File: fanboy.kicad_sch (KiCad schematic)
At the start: 51 parts, among them J1 XT30, J2 USB_C_Receptacle_USB2.0, J3 Conn_01x04, J4 Conn_01x04, SW1 GT-TC029B-H025-L1N, SW2 GT-TC029B-H025-L1N, U1 TPD1E05U06DYA, U2 TPD1E05U06DYA, U3 W25Q16JVUXIQ TR, U4 TLV1117LV33DCYR, U5 EMC2302, U6 RP2040, U7 SK6812, Y1 12MHz

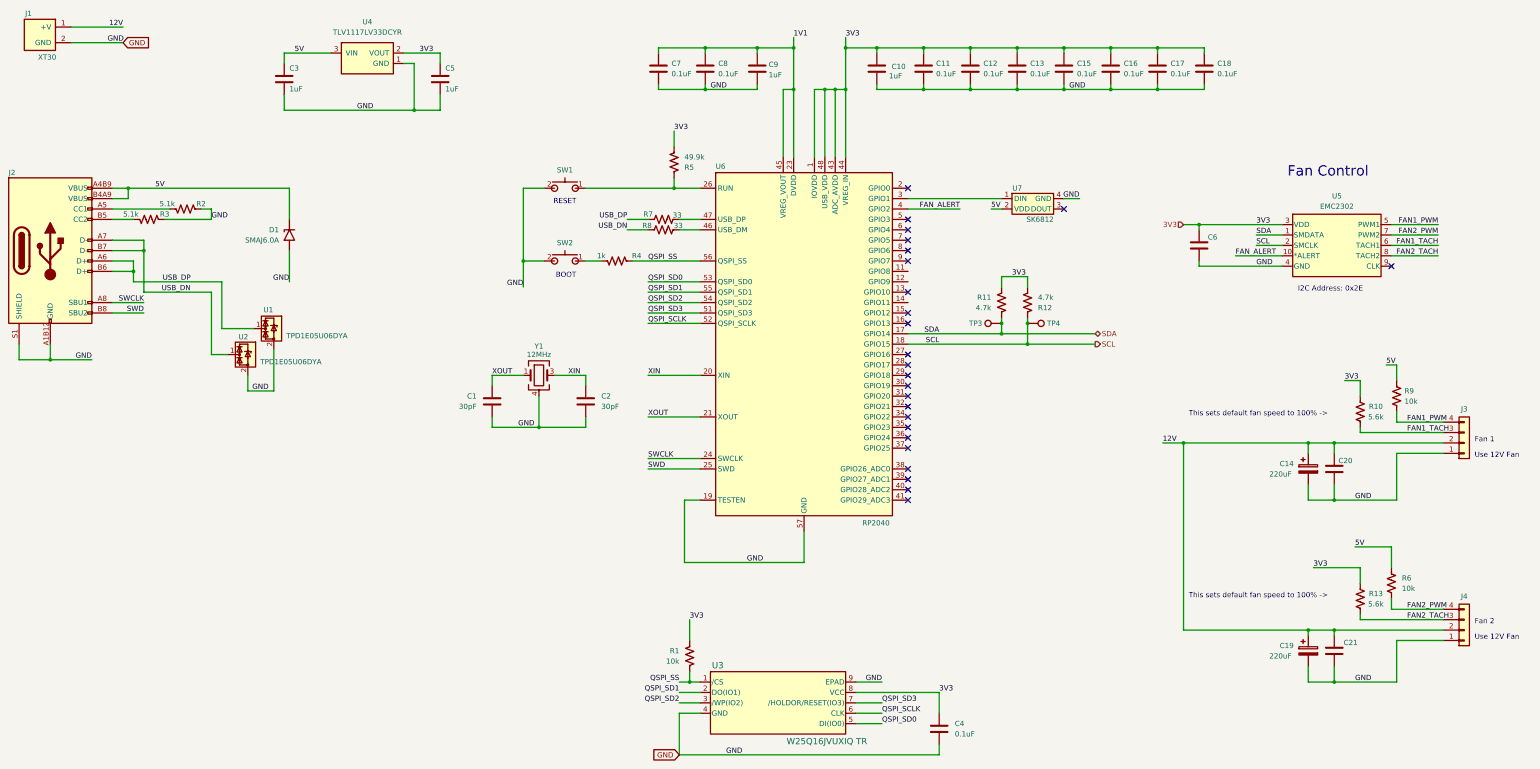
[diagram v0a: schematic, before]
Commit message: finished routing, added render and readme
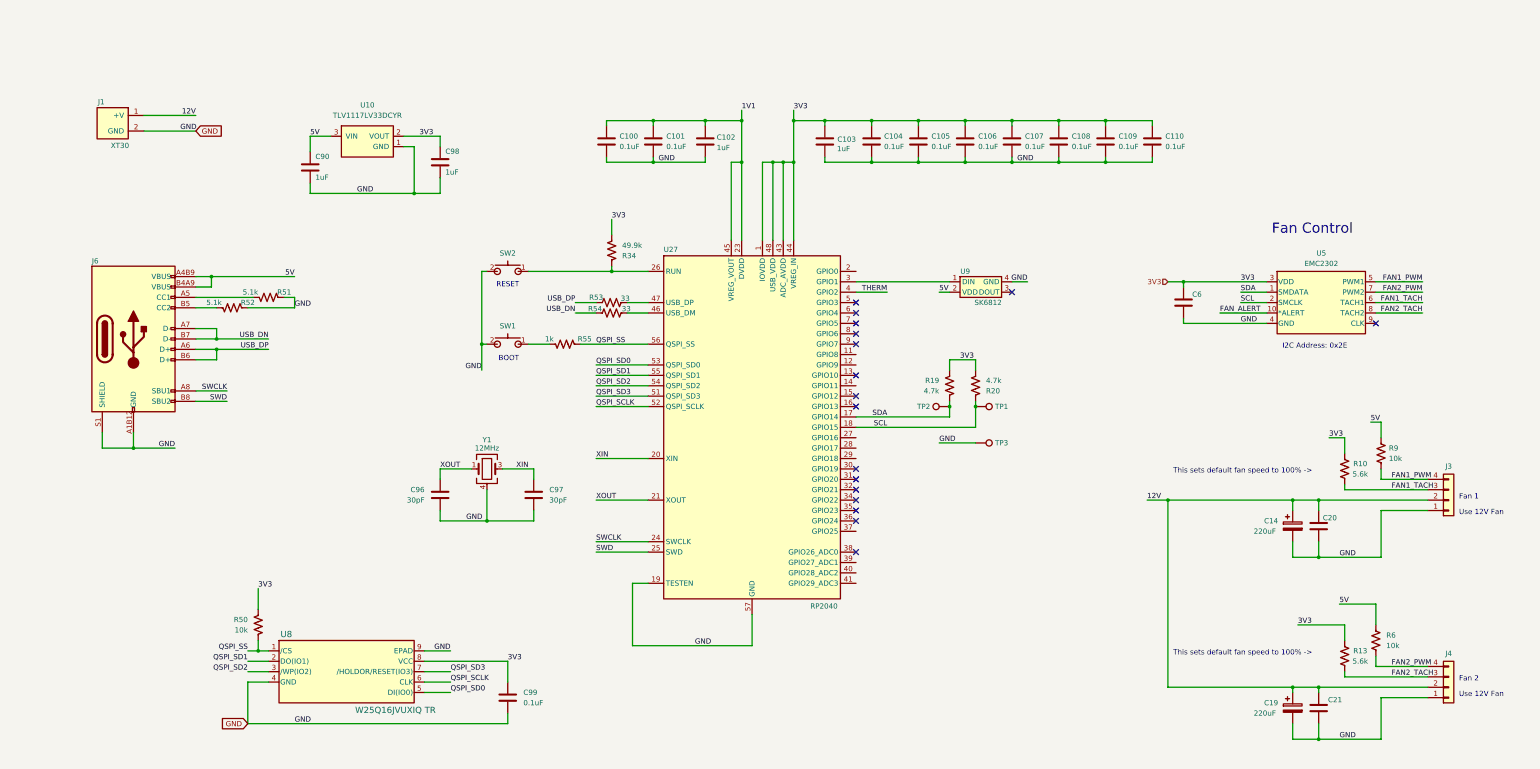
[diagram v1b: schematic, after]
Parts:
- removed C1, C2: 30pF, Capacitor_SMD:C_0402_1005Metric, symbol Device:C
- removed C10, C3, C5, C9: 1uF, Capacitor_SMD:C_0402_1005Metric, symbol Device:C
- removed C11, C12, C13, C15, C16, C17, C18, C4, C7, C8: 0.1uF, Capacitor_SMD:C_0402_1005Metric, symbol Device:C
- removed D1: SMAJ6.0A, Diode_SMD:D_SMB, symbol Diode:SMAJ6.0A
- removed J2: USB_C_Receptacle_USB2.0, aditBoard:USB_C_Receptacle_GCT_USB4105-xx-A_16P_TopMnt_Horizontal, symbol aditBoard:USB_C_Receptacle_USB2.0
- removed R1: 10k, Resistor_SMD:R_0402_1005Metric, symbol Device:R_US
- removed R11, R12: 4.7k, Resistor_SMD:R_0402_1005Metric, symbol Device:R_US
- removed R2, R3: 5.1k, Resistor_SMD:R_0402_1005Metric, symbol Device:R_US
- removed R4: 1k, Resistor_SMD:R_0402_1005Metric, symbol Device:R_US
- removed R5: 49.9k, Resistor_SMD:R_0402_1005Metric, symbol Device:R_US
- removed R7, R8: 33, Resistor_SMD:R_0402_1005Metric, symbol Device:R_US
- removed TP4: TestPoint, TestPoint:TestPoint_Pad_D1.0mm, symbol Connector:TestPoint
- removed U1, U2: TPD1E05U06DYA, Diode_SMD:D_SOD-523, symbol Power_Protection:TPD1E05U06DYA
- removed U3: W25Q16JVUXIQ TR, emberone:USON-8_UX_2x3x0p6_WIN, symbol emberone:W25Q16JVUXIQ_TR
- removed U4: TLV1117LV33DCYR, emberone:VREG_TLV1117LV33DCYR, symbol emberone:TLV1117LV33DCYR
- removed U6: RP2040, Package_DFN_QFN:QFN-56-1EP_7x7mm_P0.4mm_EP3.2x3.2mm, symbol aditBoard:RP2040
- removed U7: SK6812, emberone:LED-SMD_4P-L4.0-W1.6-L, symbol athvfd:SK6812SIDE-A-RVS
- added C100, C101, C104, C105, C106, C107, C108, C109, C110, C99: 0.1uF, Capacitor_SMD:C_0402_1005Metric, symbol Device:C
- added C102, C103, C90, C98: 1uF, Capacitor_SMD:C_0402_1005Metric, symbol Device:C
- added C96, C97: 30pF, Capacitor_SMD:C_0402_1005Metric, symbol Device:C
- added J6: USB_C_Receptacle_USB2.0, aditBoard:USB_C_Receptacle_GCT_USB4105-xx-A_16P_TopMnt_Horizontal, symbol aditBoard:USB_C_Receptacle_USB2.0
- added R19, R20: 4.7k, Resistor_SMD:R_0402_1005Metric, symbol Device:R_US
- added R34: 49.9k, Resistor_SMD:R_0402_1005Metric, symbol Device:R_US
- added R50: 10k, Resistor_SMD:R_0402_1005Metric, symbol Device:R_US
- added R51, R52: 5.1k, Resistor_SMD:R_0402_1005Metric, symbol Device:R_US
- added R53, R54: 33, Resistor_SMD:R_0402_1005Metric, symbol Device:R_US
- added R55: 1k, Resistor_SMD:R_0402_1005Metric, symbol Device:R_US
- added TP1, TP2: TestPoint, TestPoint:TestPoint_Pad_D1.0mm, symbol Connector:TestPoint
- added U10: TLV1117LV33DCYR, emberone:VREG_TLV1117LV33DCYR, symbol emberone:TLV1117LV33DCYR
- added U27: RP2040, Package_DFN_QFN:QFN-56-1EP_7x7mm_P0.4mm_EP3.2x3.2mm, symbol aditBoard:RP2040
- added U8: W25Q16JVUXIQ TR, emberone:USON-8_UX_2x3x0p6_WIN, symbol emberone:W25Q16JVUXIQ_TR
- added U9: SK6812, emberone:LED-SMD_4P-L4.0-W1.6-L, symbol athvfd:SK6812SIDE-A-RVS
- renumbered SW2 to SW1, SW1 to SW2
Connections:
- net 1V1: now also C100.2, C101.2, C102.2, U27.23 (DVDD), U27.45 (VREG_VOUT), U27.50 (DVDD)
- net 3V3: now also C103.2, C104.2, C105.2, C106.2, C107.2, C108.2, C109.2, C110.2, C98.1, C99.2, R19.1, R20.2, R34.2, R50.1, U10.2 (VOUT), U10.4 (VOUT), U27.1 (IOVDD), U27.10 (IOVDD), U27.22 (IOVDD), U27.33 (IOVDD), U27.42 (IOVDD), U27.43 (ADC_AVDD), U27.44 (VREG_IN), U27.48 (USB_VDD), U27.49 (IOVDD), U8.8 (VCC)
- net 5V: now also C90.1, J6.A4B9 (VBUS), J6.B4A9 (VBUS), U10.3 (VIN), U9.2 (VDD)
- net GND: now also TP3.1, C100.1, C101.1, C102.1, C103.1, C104.1, C105.1, C106.1, C107.1, C108.1, C109.1, C110.1, C90.2, C96.1, C97.1, C98.2, C99.1, J6.A1B12 (GND), J6.B1A12 (GND), J6.S1 (SHIELD), R51.1, R52.1, U10.1 (GND), U27.19 (TESTEN), U27.57 (GND), U8.4 (GND), U8.9 (EPAD), U9.4 (GND)
- net QSPI_SCLK: now also U27.52 (QSPI_SCLK), U8.6 (CLK)
- net QSPI_SD0: now also U27.53 (QSPI_SD0), U8.5 (DI(IO0))
- net QSPI_SD1: now also U27.55 (QSPI_SD1), U8.2 (DO(IO1))
- net QSPI_SD2: now also U27.54 (QSPI_SD2), U8.3 (/WP(IO2))
- net QSPI_SD3: now also U27.51 (QSPI_SD3), U8.7 (/HOLDOR/RESET(IO3))
- net QSPI_SS: now also R50.2, R55.1, U27.56 (QSPI_SS), U8.1 (/CS)
- net SCL: now also R20.1, TP1.1, U27.18 (GPIO15)
- net SDA: now also R19.2, TP2.1, U27.17 (GPIO14); no longer TP3.1
- net SWCLK: now also J6.A8 (SBU1), U27.24 (SWCLK)
- net SWD: now also J6.B8 (SBU2), U27.25 (SWD)
- net USB_DN: now also J6.A7 (D-), J6.B7 (D-), R54.1
- net USB_DP: now also J6.A6 (D+), J6.B6 (D+), R53.1
- net XIN: now also C97.2, U27.20 (XIN)
- net XOUT: now also C96.2, U27.21 (XOUT)
- net at SW2.1: now also R34.1, U27.26 (RUN)
- net at SW1.1: now also R55.2
- new net: R54.2, U27.46 (USB_DM)
- new net: J6.B5 (CC2), R52.2
- new net: U27.3 (GPIO1), U9.1 (DIN)
- new net: J6.A5 (CC1), R51.2
- new net: R53.2, U27.47 (USB_DP)
- new net THERM: U27.4 (GPIO2)
- no-connect marks 25 -> 17
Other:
- moved on the sheet: C14, C19, C20, C21, C6, J1, J3, J4, R10, R13, R6, R9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
